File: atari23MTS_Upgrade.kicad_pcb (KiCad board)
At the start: 2 copper layers, 136 x 88 mm, 71 parts, among them P1 CONN_01X01, P2 CONN_01X01, P3 CONN_01X01, P4 CONN_01X01, P5 CONN_01X01, P6 CONN_01X01, SW1 SW_PUSH, U1 NCP1117ST33T3G, U10 TXB0108-PW, U11 ISSI61WV5128BL, U12 ISSI61WV5128BL, U13 ISSI61WV5128BL, U14 ISSI61WV5128BL, U15 74LS08, U16 74LS08, U2 STM32F401RCTx, U3 74LS138, U4 TXB0108-PW, U5 TXB0108-PW, U6 TXB0108-PW, U7 74HC04, U8 TXB0108-PW, U9 74LS32

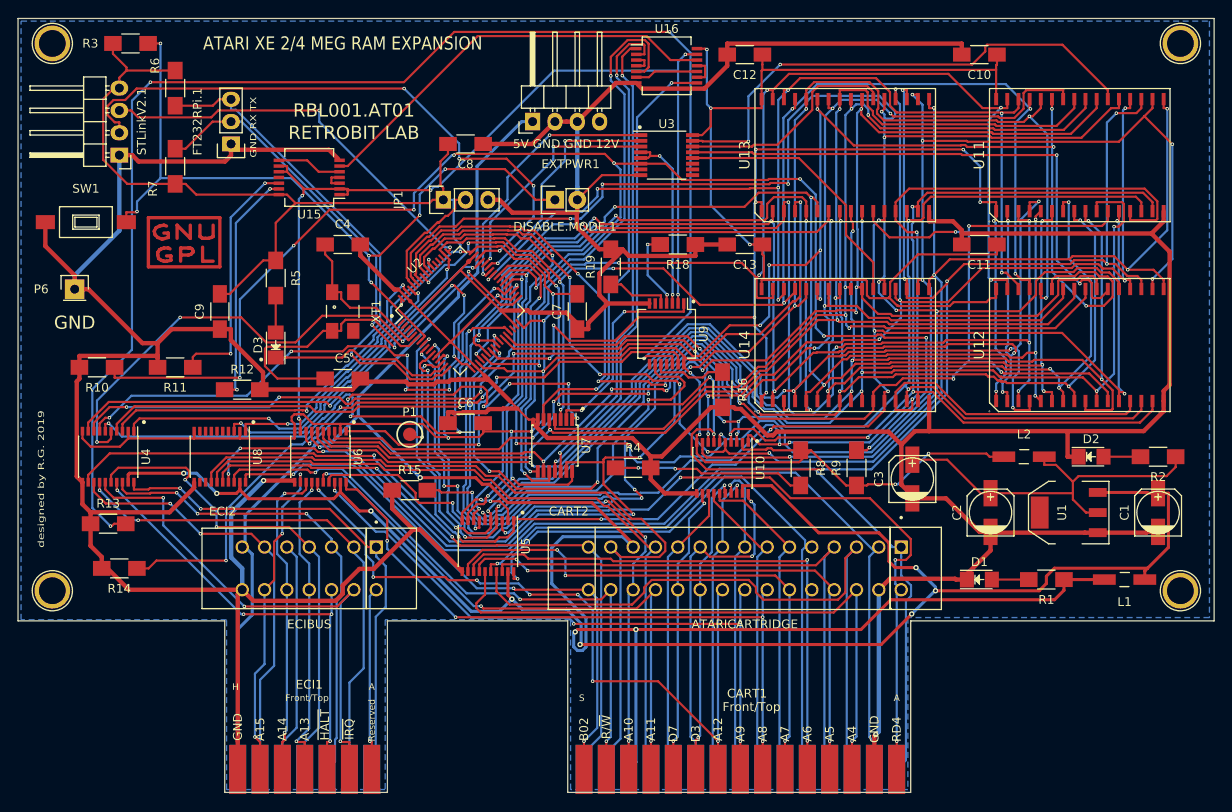
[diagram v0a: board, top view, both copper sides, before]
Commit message: Transformation will begin shortly... ;-)
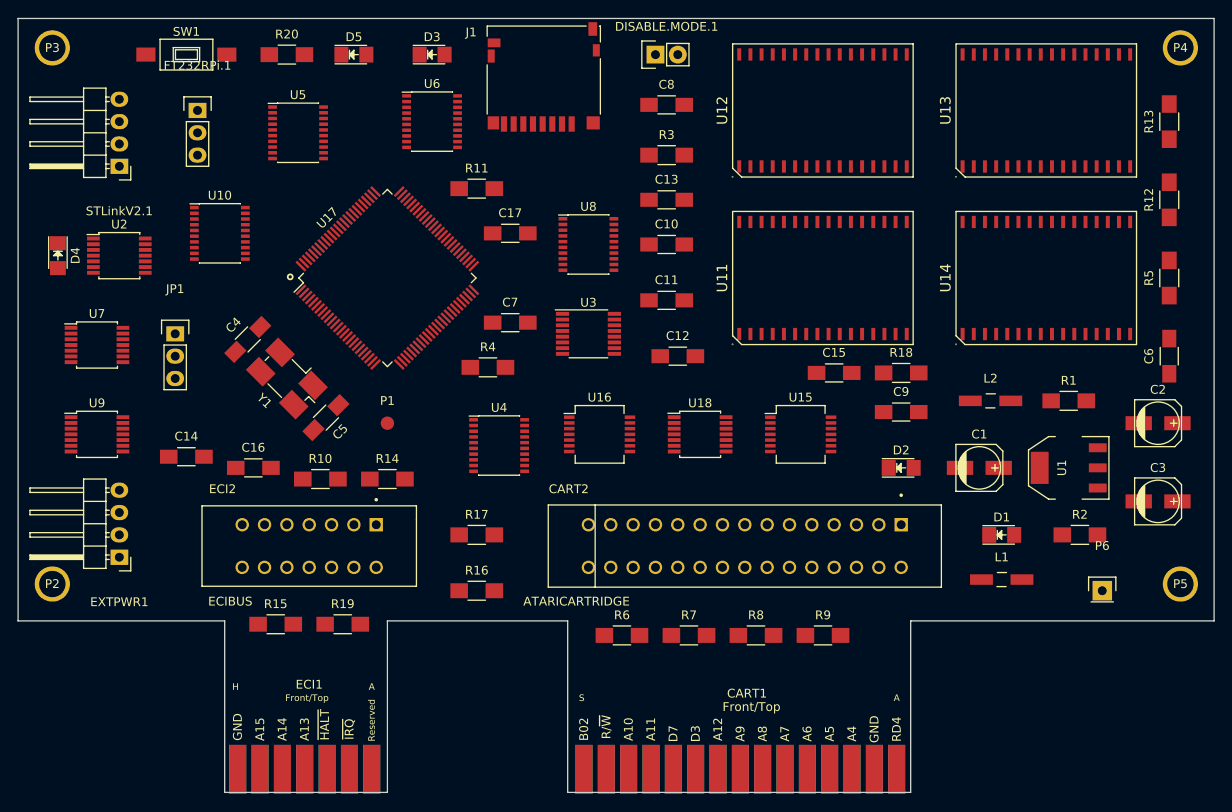
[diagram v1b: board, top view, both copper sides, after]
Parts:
- removed G***: LOGO, RetroBitLab:atari_fuji_SilkScreen_21.2x25-Rev
- removed REF**: Symbol_GNU-GPL_CopperTop_Small, Symbols:Symbol_GNU-GPL_CopperTop_Small
- removed XT1: 8Mhz, Crystals:Crystal_SMD_0603_4Pads
- added C14: 100n, Capacitors_SMD:C_1206_HandSoldering, F.Cu at (104.1, 100.3)
- added C15: 100n, Capacitors_SMD:C_1206_HandSoldering, F.Cu at (177.8, 90.8)
- added C16: 100n, Capacitors_SMD:C_1206_HandSoldering, F.Cu at (111.8, 101.6)
- added C17: 100n, Capacitors_SMD:C_1206_HandSoldering, F.Cu at (141.0, 74.9)
- added D4: LED.AMBER, LEDs:LED_1206, F.Cu at (89.5, 77.5)
- added D5: LED.RED, LEDs:LED_1206, F.Cu at (123.2, 54.6)
- added J1: Micro_SD_Card_Det, RetroBitLab:microSD_HC_Hirose_DM3D-SF, F.Cu at (144.8, 57.1)
- added R17: 0, Resistors_SMD:R_1206_HandSoldering, F.Cu at (137.2, 109.2)
- added R20: 220, Resistors_SMD:R_1206_HandSoldering, F.Cu at (115.6, 54.6)
- added U17: STM32F407VETx, Housings_QFP:LQFP-100_14x14mm_Pitch0.5mm, F.Cu at (127.0, 80.0)
- added U18: 74LS08, Housings_SSOP:TSSOP-14_4.4x5mm_Pitch0.65mm, F.Cu at (162.6, 97.8)
- added Y1: 8Mhz, Crystal:Crystal_SMD_0603-4Pin_6.0x3.5mm_HandSoldering, F.Cu at (115.6, 91.4)
- C4, C5: value C_Small -> 20p
- CART1: footprint ATARI-LEFT-CARTRIDGE -> RetroBitLab:ATARI-LEFT-CARTRIDGE
- D3: value ACT -> LED.GREEN
- P2, P3, P4, P5: footprint Connect:1pin -> RetroBitLab:MountingHole
- R10, R4: value 2.2k -> 220
- R11, R12: value 0 -> 10k
- R18: value 0 -> 47k
- R6, R7, R8, R9: value 10K -> 0
- U2: value STM32F401RCTx -> 74HC04; footprint Housings_QFP:LQFP-64_10x10mm_Pitch0.5mm -> Housings_SSOP:TSSOP-14_4.4x5mm_Pitch0.65mm
- U9: value 74LS32 -> 74HC04; footprint Housings_SSOP:SSOP-14_5.3x6.2mm_Pitch0.65mm -> Housings_SSOP:TSSOP-14_4.4x5mm_Pitch0.65mm
- moved R13 129.0 mm to (215.9, 62.2), turned to 90 degrees
- moved P6 121.8 mm to (208.3, 115.6)
- moved R12 107.6 mm to (215.9, 71.1), turned to 90 degrees
- moved R5 101.6 mm to (215.9, 80.0), turned to 90 degrees
- moved C6 80.4 mm to (215.9, 88.9), turned to 90 degrees
- moved R6 80.3 mm to (153.7, 120.7), turned to 0 degrees
- moved R7 79.1 mm to (161.3, 120.7), turned to 0 degrees
- moved C9 78.3 mm to (185.4, 95.2), turned to 0 degrees
- moved EXTPWR1 68.3 mm to (96.5, 111.8), turned to 180 degrees
- moved U9 65.8 mm to (94.0, 97.8), turned to 0 degrees
- moved U10 63.1 mm to (108.0, 74.9), turned to 0 degrees
- moved U15 63.1 mm to (174.0, 97.8), turned to 0 degrees
- moved R3 62.3 mm to (158.8, 66.0), turned to 0 degrees
- moved U7 53.3 mm to (94.0, 87.6), turned to 0 degrees
- moved U5 51.7 mm to (116.8, 63.5), turned to 0 degrees
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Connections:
- D3 pad 1: Net-(D3-Pad1) -> GND
- EXTPWR1 pad 4: Net-(EXTPWR1-Pad4) -> (no net)
- P2 pad 1: Net-(P2-Pad1) -> (no net)
- P3 pad 1: Net-(P3-Pad1) -> (no net)
- P4 pad 1: Net-(P4-Pad1) -> (no net)
- P5 pad 1: Net-(P5-Pad1) -> (no net)
- R10 pad 1: RAMEN -> Net-(D5-Pad2)
- R10 pad 2: GND -> LEDRED
- R11 pad 1: Net-(R11-Pad1) -> VCC3V3
- R11 pad 2: GND -> UART_RX_TTL
- R12 pad 1: Net-(R12-Pad1) -> VCC3V3
- R12 pad 2: GND -> UART_TX_TTL
- R13 pad 2: Net-(R13-Pad2) -> /MCU/SPARE1
- R14 pad 1: Net-(R14-Pad1) -> GND
- R14 pad 2: GND -> /MCU/SPARE2
- R15 pad 2: Net-(R15-Pad2) -> /MCU/SPARE3
- R16 pad 1: Net-(R16-Pad1) -> GND
- R16 pad 2: GND -> /MCU/SPARE4
- R18 pad 1: GND -> VCC3V3
- R18 pad 2: Net-(R18-Pad2) -> mSDO
- R19 pad 2: GND -> Net-(C4-Pad1)
- R4 pad 1: Net-(R4-Pad1) -> Net-(D3-Pad2)
- R4 pad 2: GND -> LEDGRN
- R5 pad 1: VCC3V3 -> Net-(D4-Pad2)
- R5 pad 2: Net-(D3-Pad2) -> LEDAMBER
- R6 pad 1: VCC3V3 -> GND
- R6 pad 2: UART_TX_TTL -> Net-(R6-Pad2)
- R7 pad 1: VCC3V3 -> GND
- R7 pad 2: UART_RX_TTL -> Net-(R7-Pad2)
- R8 pad 1: VCC3V3 -> GND
- R8 pad 2: Net-(R4-Pad1) -> Net-(R8-Pad2)
- R9 pad 1: VCC3V3 -> GND
- R9 pad 2: RAMEN -> Net-(R9-Pad2)
- U11 pad 1: PB3 -> mD1E2_A17
- U11 pad 2: PB2 -> mD1E2_A16
- U11 pad 23: mA10 -> mD1E0_A10
- U11 pad 25: mA11 -> mD1E0_A11
- U11 pad 26: mA9 -> mD1E0_A9
- U11 pad 27: mA8 -> mD1E0_A8
- U11 pad 28: mA13 -> mD1E0_A13
- U11 pad 3: PB0 -> mD1E0_A14
- U11 pad 30: PB4 -> mD1E2_A18
- U11 pad 31: PB1 -> mD1E0_A15
- U11 pad 4: mA12 -> mD1E0_A12
- U12 pad 1: PB3 -> mD1E2_A17
- U12 pad 2: PB2 -> mD1E2_A16
- U12 pad 23: mA10 -> mD1E0_A10
- U12 pad 25: mA11 -> mD1E0_A11
- U12 pad 26: mA9 -> mD1E0_A9
- U12 pad 27: mA8 -> mD1E0_A8
- U12 pad 28: mA13 -> mD1E0_A13
- U12 pad 3: PB0 -> mD1E0_A14
- U12 pad 30: PB4 -> mD1E2_A18
- U12 pad 31: PB1 -> mD1E0_A15
- U12 pad 4: mA12 -> mD1E0_A12
- U13 pad 1: PB3 -> mD1E2_A17
- U13 pad 2: PB2 -> mD1E2_A16
- U13 pad 23: mA10 -> mD1E0_A10
- U13 pad 25: mA11 -> mD1E0_A11
- U13 pad 26: mA9 -> mD1E0_A9
- U13 pad 27: mA8 -> mD1E0_A8
- U13 pad 28: mA13 -> mD1E0_A13
- U13 pad 3: PB0 -> mD1E0_A14
- U13 pad 30: PB4 -> mD1E2_A18
- U13 pad 31: PB1 -> mD1E0_A15
- U13 pad 4: mA12 -> mD1E0_A12
- U14 pad 1: PB3 -> mD1E2_A17
- U14 pad 2: PB2 -> mD1E2_A16
- U14 pad 23: mA10 -> mD1E0_A10
- U14 pad 25: mA11 -> mD1E0_A11
- U14 pad 26: mA9 -> mD1E0_A9
- U14 pad 27: mA8 -> mD1E0_A8
- U14 pad 28: mA13 -> mD1E0_A13
- U14 pad 3: PB0 -> mD1E0_A14
- U14 pad 30: PB4 -> mD1E2_A18
- U14 pad 31: PB1 -> mD1E0_A15
- U14 pad 4: mA12 -> mD1E0_A12
- U15 pad 10: mA15 -> ~mA13
- U15 pad 11: Net-(U15-Pad11) -> ~mA11mA9
- U15 pad 12: Net-(R11-Pad1) -> ~mA11
- U15 pad 13: Net-(R12-Pad1) -> mA9
- U15 pad 2: mA15 -> mA14
- U15 pad 5: Net-(U15-Pad5) -> mA12
- U15 pad 8: Net-(U15-Pad5) -> mDXXX
- U15 pad 9: mA15 -> Net-(U15-Pad6)
- U16 pad 1: ~mA13 -> mA10
- U16 pad 10: Net-(U16-Pad10) -> mA8
- U16 pad 11: Net-(U16-Pad11) -> mX6XX
- U16 pad 12: Net-(U15-Pad6) -> Net-(U16-Pad12)
- U16 pad 13: mA15 -> ~mA11mA9
- U16 pad 2: ~mA11 -> ~mA8
- U16 pad 3: Net-(U16-Pad3) -> Net-(U16-Pad12)
- U16 pad 4: Net-(U16-Pad3) -> ~mA11mA9
- U16 pad 5: ~mA10 -> Net-(U16-Pad5)
- U16 pad 6: Net-(U16-Pad10) -> mX3XX
- U16 pad 8: mD3XX -> Net-(U16-Pad5)
- U16 pad 9: Net-(U16-Pad11) -> ~mA10
- U2 pad 1: Net-(U2-Pad1) -> (no net)
- U2 pad 10: mA2 -> (no net)
- U2 pad 11: mA3 -> (no net)
- U2 pad 12: GND -> (no net)
- U2 pad 13: VCC3V3 -> (no net)
- U2 pad 14: TP1 -> VCC3V3
- U2 pad 2: Net-(U2-Pad2) -> (no net)
- U2 pad 3: Net-(U2-Pad3) -> (no net)
- U2 pad 4: Net-(U2-Pad4) -> (no net)
- U2 pad 5: Net-(C4-Pad1) -> (no net)
- U2 pad 6: Net-(C5-Pad1) -> (no net)
- U2 pad 7: nRESET -> GND
- U2 pad 8: mA0 -> (no net)
- U2 pad 9: mA1 -> (no net)
- U3 pad 1: PB5 -> mD1E2_A19
- U3 pad 10: Net-(U3-Pad10) -> (no net)
- U3 pad 11: Net-(U3-Pad11) -> (no net)
- U3 pad 2: PB6 -> mD1E3_A20
- U3 pad 3: PB7 -> mD1E3_A21
- U3 pad 4: ~ADDRSEL16K -> ~mD6XX
- U3 pad 5: ~ADDRSEL16K -> ~mD6XX
- U3 pad 7: Net-(U3-Pad7) -> (no net)
- U3 pad 9: Net-(U3-Pad9) -> (no net)
- U7 pad 1: mA14 -> mA10
- U7 pad 2: Net-(U7-Pad2) -> ~mA10
- U7 pad 8: ~mA10 -> ~mA8
- U7 pad 9: mA10 -> mA8
- U8 pad 12: Net-(U8-Pad12) -> (no net)
- U8 pad 13: Net-(U8-Pad13) -> (no net)
- U8 pad 8: Net-(U8-Pad8) -> (no net)
- U8 pad 9: Net-(U8-Pad9) -> (no net)
- U9 pad 1: Net-(U7-Pad2) -> mD6XX
- U9 pad 10: Net-(R16-Pad1) -> (no net)
- U9 pad 11: Net-(U9-Pad11) -> (no net)
- U9 pad 12: Net-(R13-Pad2) -> (no net)
- U9 pad 13: Net-(R14-Pad1) -> (no net)
- U9 pad 14: VCC3V3 -> (no net)
- U9 pad 2: mA15 -> ~mD6XX
- U9 pad 3: ~ADDRSEL16K -> (no net)
- U9 pad 4: Net-(R18-Pad2) -> (no net)
- U9 pad 5: Net-(R19-Pad1) -> (no net)
- U9 pad 6: Net-(U9-Pad6) -> (no net)
- U9 pad 7: GND -> (no net)
- U9 pad 8: Net-(U9-Pad8) -> (no net)
- U9 pad 9: Net-(R15-Pad2) -> (no net)
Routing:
- net GND: track 691.0 -> 0.00 mm, vias 2 -> 0
- net VCC3V3: track 466.9 -> 0.00 mm, vias 19 -> 0
- net +5VDC: track 234.2 -> 0.00 mm, vias 3 -> 0
- net mD7: track 200.4 -> 0.00 mm, vias 9 -> 0
- net mD5: track 189.0 -> 0.00 mm, vias 12 -> 0
- net mD4: track 188.6 -> 0.00 mm, vias 9 -> 0
- net mA1: track 186.7 -> 0.00 mm, vias 11 -> 0
- net VCC5V: track 186.2 -> 0.00 mm, vias 8 -> 0
- net mD0: track 183.2 -> 0.00 mm, vias 5 -> 0
- net mR/~W: track 176.9 -> 0.00 mm, vias 9 -> 0
- net mA13: track 171.9 -> 0.00 mm, vias 8 -> 0
- net mD3: track 170.7 -> 0.00 mm, vias 9 -> 0
- net RAMEN: track 170.4 -> 0.00 mm, vias 10 -> 0
- net mD6: track 168.4 -> 0.00 mm, vias 10 -> 0
- net mA3: track 166.6 -> 0.00 mm, vias 8 -> 0
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- removed copper zone on B.Cu, net GND
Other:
- board text removed: "5V GND GND 12V"
- board text removed: "8-BIT"
- board text removed: "ATARI XE 2/4 MEG RAM EXPANSION"
- board text removed: "GND"
- board text removed: "GND RX TX"
- board text removed: "Power Without the Price!"
- board text removed: "RBL001.AT01"
- board text removed: "RETROBIT LAB"
- board text removed: "designed by R.G. 2019"
- board text removed: "in memoriam A.S.-G.D."
